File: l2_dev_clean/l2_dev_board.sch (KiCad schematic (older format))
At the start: 46 parts

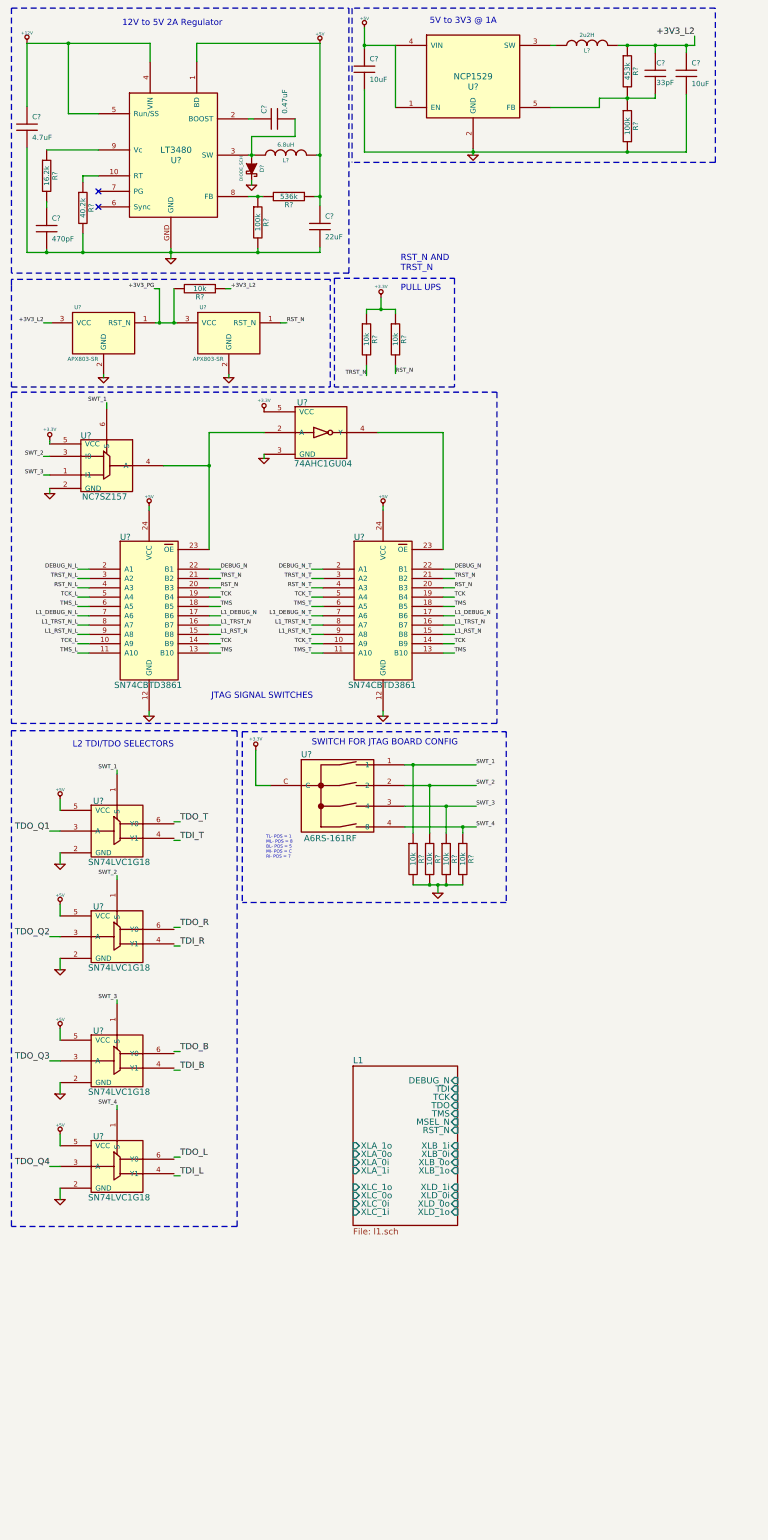
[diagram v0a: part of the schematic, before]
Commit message: added a buffer for reverse L1 but has an empty line, Might buffer in 2 directions!
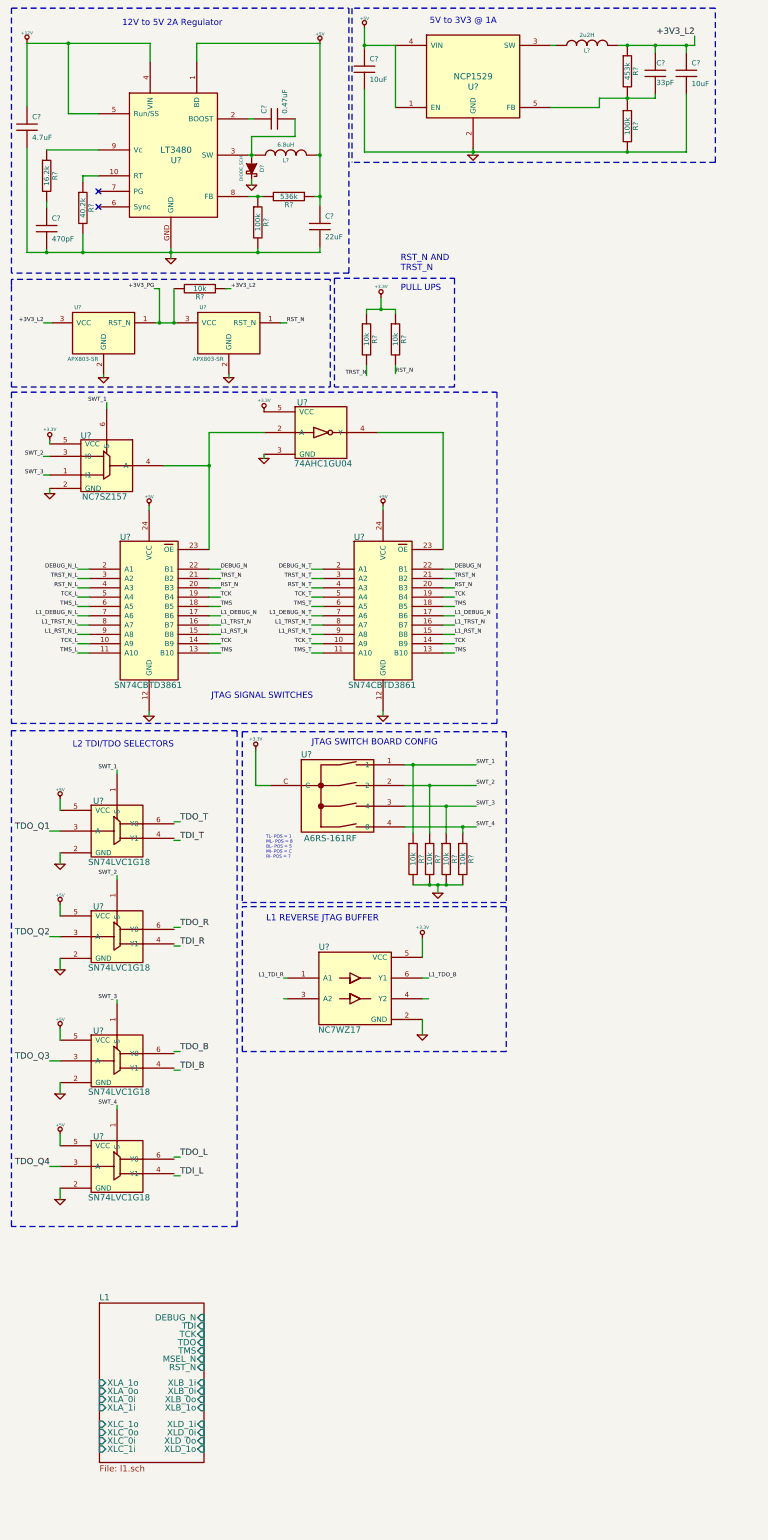
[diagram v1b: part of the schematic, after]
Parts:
- added U?: NC7WZ17, symbol NC7WZ17
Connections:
- net L2_PAIR/BL_X0_XLA_0i is gone; now on net L2_PAIR/BL_X0_XLA_0i: P?.7 (P7)
- net L2_PAIR/BL_X0_XLA_0o is gone; now on net L2_PAIR/BL_X0_XLA_0o: P?.10 (P10)
- net L2_PAIR/BL_X0_XLA_1i is gone; now on net L2_PAIR/BL_X0_XLA_1i: P?.6 (P6)
- net L2_PAIR/BL_X0_XLA_1o is gone; now on net L2_PAIR/BL_X0_XLA_1o: P?.11 (P11)
- net L2_PAIR/BL_X0_XLA_2i is gone; now on net L2_PAIR/BL_X0_XLA_2i: P?.5 (P5)
- net L2_PAIR/BL_X0_XLA_2o is gone; now on net L2_PAIR/BL_X0_XLA_2o: P?.12 (P12)
- net L2_PAIR/BL_X0_XLA_3i is gone; now on net L2_PAIR/BL_X0_XLA_3i: P?.4 (P4)
- net L2_PAIR/BL_X0_XLA_3o is gone; now on net L2_PAIR/BL_X0_XLA_3o: P?.13 (P13)
- net L2_PAIR/BL_X0_XLA_4i is gone; now on net L2_PAIR/BL_X0_XLA_4i: P?.3 (P3)
- net L2_PAIR/BL_X0_XLA_4o is gone; now on net L2_PAIR/BL_X0_XLA_4o: P?.14 (P14)
- net L2_PAIR/BR_X1_XLA_0i is gone; now on net L2_PAIR/BR_X1_XLA_0i: P?.9 (P9)
- net L2_PAIR/BR_X1_XLA_0o is gone; now on net L2_PAIR/BR_X1_XLA_0o: P?.6 (P6)
- net L2_PAIR/BR_X1_XLA_1i is gone; now on net L2_PAIR/BR_X1_XLA_1i: P?.10 (P10)
- net L2_PAIR/BR_X1_XLA_1o is gone; now on net L2_PAIR/BR_X1_XLA_1o: P?.5 (P5)
- net L2_PAIR/BR_X1_XLA_2i is gone; now on net L2_PAIR/BR_X1_XLA_2i: P?.11 (P11)
- net L2_PAIR/BR_X1_XLA_2o is gone; now on net L2_PAIR/BR_X1_XLA_2o: P?.4 (P4)
- net L2_PAIR/BR_X1_XLA_3i is gone; now on net L2_PAIR/BR_X1_XLA_3i: P?.2 (P2)
- net L2_PAIR/BR_X1_XLA_3o is gone; now on net L2_PAIR/BR_X1_XLA_3o: P?.3 (P3)
- net L2_PAIR/BR_X1_XLA_4i is gone; now on net L2_PAIR/BR_X1_XLA_4i: P?.3 (P3)
- net L2_PAIR/BR_X1_XLA_4o is gone; now on net L2_PAIR/BR_X1_XLA_4o: P?.2 (P2)
- net L2_PAIR/B_X1_XLB_0i is gone; now on net L2_PAIR/B_X1_XLB_0i: P?.7 (P7)
- net L2_PAIR/B_X1_XLB_0o is gone; now on net L2_PAIR/B_X1_XLB_0o: P?.24 (P24)
- net L2_PAIR/B_X1_XLB_1i is gone; now on net L2_PAIR/B_X1_XLB_1i: P?.6 (P6)
- net L2_PAIR/B_X1_XLB_1o is gone; now on net L2_PAIR/B_X1_XLB_1o: P?.25 (P25)
- net L2_PAIR/B_X1_XLB_2i is gone; now on net L2_PAIR/B_X1_XLB_2i: P?.5 (P5)
- net L2_PAIR/B_X1_XLB_2o is gone; now on net L2_PAIR/B_X1_XLB_2o: P?.26 (P26)
- net L2_PAIR/B_X1_XLB_3i is gone; now on net L2_PAIR/B_X1_XLB_3i: P?.4 (P4)
- net L2_PAIR/B_X1_XLB_3o is gone; now on net L2_PAIR/B_X1_XLB_3o: P?.27 (P27)
- net L2_PAIR/B_X1_XLB_4i is gone; now on net L2_PAIR/B_X1_XLB_4i: P?.3 (P3)
- net L2_PAIR/B_X1_XLB_4o is gone; now on net L2_PAIR/B_X1_XLB_4o: P?.28 (P28)
- net L2_PAIR/TL_X0_XLA_0i is gone; now on net L2_PAIR/TL_X0_XLA_0i: P?.21 (P21)
- net L2_PAIR/TL_X0_XLA_0o is gone; now on net L2_PAIR/TL_X0_XLA_0o: P?.24 (P24)
- net L2_PAIR/TL_X0_XLA_1i is gone; now on net L2_PAIR/TL_X0_XLA_1i: P?.20 (P20)
- net L2_PAIR/TL_X0_XLA_1o is gone; now on net L2_PAIR/TL_X0_XLA_1o: P?.25 (P25)
- net L2_PAIR/TL_X0_XLA_2i is gone; now on net L2_PAIR/TL_X0_XLA_2i: P?.19 (P19)
- net L2_PAIR/TL_X0_XLA_2o is gone; now on net L2_PAIR/TL_X0_XLA_2o: P?.26 (P26)
- net L2_PAIR/TL_X0_XLA_3i is gone; now on net L2_PAIR/TL_X0_XLA_3i: P?.18 (P18)
- net L2_PAIR/TL_X0_XLA_3o is gone; now on net L2_PAIR/TL_X0_XLA_3o: P?.27 (P27)
- net L2_PAIR/TL_X0_XLA_4i is gone; now on net L2_PAIR/TL_X0_XLA_4i: P?.17 (P17)
- net L2_PAIR/TL_X0_XLA_4o is gone; now on net L2_PAIR/TL_X0_XLA_4o: P?.28 (P28)
- net L2_PAIR/TR_X1_XLA_0i is gone; now on net L2_PAIR/TR_X1_XLA_0i: P?.13 (P13)
- net L2_PAIR/TR_X1_XLA_0o is gone; now on net L2_PAIR/TR_X1_XLA_0o: P?.10 (P10)
- net L2_PAIR/TR_X1_XLA_1i is gone; now on net L2_PAIR/TR_X1_XLA_1i: P?.14 (P14)
- net L2_PAIR/TR_X1_XLA_1o is gone; now on net L2_PAIR/TR_X1_XLA_1o: P?.9 (P9)
- net L2_PAIR/TR_X1_XLA_2i is gone; now on net L2_PAIR/TR_X1_XLA_2i: P?.15 (P15)
- net L2_PAIR/TR_X1_XLA_2o is gone; now on net L2_PAIR/TR_X1_XLA_2o: P?.8 (P8)
- net L2_PAIR/TR_X1_XLA_3i is gone; now on net L2_PAIR/TR_X1_XLA_3i: P?.16 (P16)
- net L2_PAIR/TR_X1_XLA_3o is gone; now on net L2_PAIR/TR_X1_XLA_3o: P?.7 (P7)
- net L2_PAIR/TR_X1_XLA_4i is gone; now on net L2_PAIR/TR_X1_XLA_4i: P?.17 (P17)
- net L2_PAIR/TR_X1_XLA_4o is gone; now on net L2_PAIR/TR_X1_XLA_4o: P?.6 (P6)
- net L2_PAIR/T_X0_XLB_0i is gone; now on net L2_PAIR/T_X0_XLB_0i: P?.7 (P7)
- net L2_PAIR/T_X0_XLB_0o is gone; now on net L2_PAIR/T_X0_XLB_0o: P?.24 (P24)
- net L2_PAIR/T_X0_XLB_1i is gone; now on net L2_PAIR/T_X0_XLB_1i: P?.6 (P6)
- net L2_PAIR/T_X0_XLB_1o is gone; now on net L2_PAIR/T_X0_XLB_1o: P?.25 (P25)
- net L2_PAIR/T_X0_XLB_2i is gone; now on net L2_PAIR/T_X0_XLB_2i: P?.5 (P5)
- net L2_PAIR/T_X0_XLB_2o is gone; now on net L2_PAIR/T_X0_XLB_2o: P?.26 (P26)
- net L2_PAIR/T_X0_XLB_3i is gone; now on net L2_PAIR/T_X0_XLB_3i: P?.4 (P4)
- net L2_PAIR/T_X0_XLB_3o is gone; now on net L2_PAIR/T_X0_XLB_3o: P?.27 (P27)
- net L2_PAIR/T_X0_XLB_4i is gone; now on net L2_PAIR/T_X0_XLB_4i: P?.3 (P3)
- net L2_PAIR/T_X0_XLB_4o is gone; now on net L2_PAIR/T_X0_XLB_4o: P?.28 (P28)
- net +3.3V: now also U?.5 (VCC)
- net GND: now also U?.2 (GND)
- net L1_TDI_R: now also U?.1 (A1)
- net L1_TDO_B: now also U?.6 (Y1)
- net L2_PAIR/BR_X1_XLA_0i: no longer P?.10 (P10)
- net L2_PAIR/BR_X1_XLA_0o: no longer P?.7 (P7)
- net L2_PAIR/BR_X1_XLA_1i: no longer P?.11 (P11)
- net L2_PAIR/BR_X1_XLA_1o: no longer P?.6 (P6)
- net L2_PAIR/BR_X1_XLA_2i: no longer P?.12 (P12)
- net L2_PAIR/BR_X1_XLA_2o: no longer P?.5 (P5)
- net L2_PAIR/BR_X1_XLA_3i: no longer P?.13 (P13)
- net L2_PAIR/BR_X1_XLA_3o: no longer P?.4 (P4)
- net L2_PAIR/BR_X1_XLA_4i: no longer P?.14 (P14)
- net L2_PAIR/BR_X1_XLA_4o: no longer P?.3 (P3)
- net L2_PAIR/TR_X1_XLA_0i: no longer P?.24 (P24)
- net L2_PAIR/TR_X1_XLA_0o: no longer P?.21 (P21)
- net L2_PAIR/TR_X1_XLA_1i: no longer P?.25 (P25)
- net L2_PAIR/TR_X1_XLA_1o: no longer P?.20 (P20)
- net L2_PAIR/TR_X1_XLA_2i: no longer P?.26 (P26)
- net L2_PAIR/TR_X1_XLA_2o: no longer P?.19 (P19)
- net L2_PAIR/TR_X1_XLA_3i: no longer P?.27 (P27)
- net L2_PAIR/TR_X1_XLA_3o: no longer P?.18 (P18)
- net L2_PAIR/TR_X1_XLA_4i: no longer P?.28 (P28)
- net L2_PAIR/TR_X1_XLA_4o: no longer P?.17 (P17)
- net L2_PAIR/T_X0_XLB_0i: no longer P?.21 (P21)
- net L2_PAIR/T_X0_XLB_0o: no longer P?.10 (P10)
- net L2_PAIR/T_X0_XLB_1i: no longer P?.20 (P20)
- net L2_PAIR/T_X0_XLB_1o: no longer P?.11 (P11)
- net L2_PAIR/T_X0_XLB_2i: no longer P?.19 (P19)
- net L2_PAIR/T_X0_XLB_2o: no longer P?.12 (P12)
- net L2_PAIR/T_X0_XLB_3i: no longer P?.18 (P18)
- net L2_PAIR/T_X0_XLB_3o: no longer P?.13 (P13)
- net L2_PAIR/T_X0_XLB_4i: no longer P?.17 (P17)
- net L2_PAIR/T_X0_XLB_4o: no longer P?.14 (P14)
- new net L2_PAIR/BR_X1_XLA_0i: P?.10 (P10)
- new net L2_PAIR/BR_X1_XLA_0o: P?.7 (P7)
- new net L2_PAIR/BR_X1_XLA_1i: P?.11 (P11)
- new net L2_PAIR/BR_X1_XLA_1o: P?.6 (P6)
- new net L2_PAIR/BR_X1_XLA_2i: P?.12 (P12)
- new net L2_PAIR/BR_X1_XLA_2o: P?.5 (P5)
- new net L2_PAIR/BR_X1_XLA_3i: P?.13 (P13)
- new net L2_PAIR/BR_X1_XLA_3o: P?.4 (P4)
- new net L2_PAIR/BR_X1_XLA_4i: P?.14 (P14)
- new net L2_PAIR/BR_X1_XLA_4o: P?.3 (P3)
- new net L2_PAIR/TR_X1_XLA_0i: P?.24 (P24)
- new net L2_PAIR/TR_X1_XLA_0o: P?.21 (P21)
- new net L2_PAIR/TR_X1_XLA_1i: P?.25 (P25)
- new net L2_PAIR/TR_X1_XLA_1o: P?.20 (P20)
- new net L2_PAIR/TR_X1_XLA_2i: P?.26 (P26)
- new net L2_PAIR/TR_X1_XLA_2o: P?.19 (P19)
- new net L2_PAIR/TR_X1_XLA_3i: P?.27 (P27)
- new net L2_PAIR/TR_X1_XLA_3o: P?.18 (P18)
- new net L2_PAIR/TR_X1_XLA_4i: P?.28 (P28)
- new net L2_PAIR/TR_X1_XLA_4o: P?.17 (P17)
- new net L2_PAIR/T_X0_XLB_0i: P?.21 (P21)
- new net L2_PAIR/T_X0_XLB_0o: P?.10 (P10)
- new net L2_PAIR/T_X0_XLB_1i: P?.20 (P20)
- new net L2_PAIR/T_X0_XLB_1o: P?.11 (P11)
- new net L2_PAIR/T_X0_XLB_2i: P?.19 (P19)
- new net L2_PAIR/T_X0_XLB_2o: P?.12 (P12)
- new net L2_PAIR/T_X0_XLB_3i: P?.18 (P18)
- new net L2_PAIR/T_X0_XLB_3o: P?.13 (P13)
- new net L2_PAIR/T_X0_XLB_4i: P?.17 (P17)
- new net L2_PAIR/T_X0_XLB_4o: P?.14 (P14)
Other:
- note added: "JTAG SWITCH BOARD CONFIG"
- note added: "L1 REVERSE JTAG BUFFER"
- note removed: "SWITCH FOR JTAG BOARD CONFIG"
